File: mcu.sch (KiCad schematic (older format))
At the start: 28 parts, among them P1 CONN_01X02, SW1 SW_PUSH, T2 MMBT3904, U2 STM32F072CB, U6 24AA01, Y1 8MHz

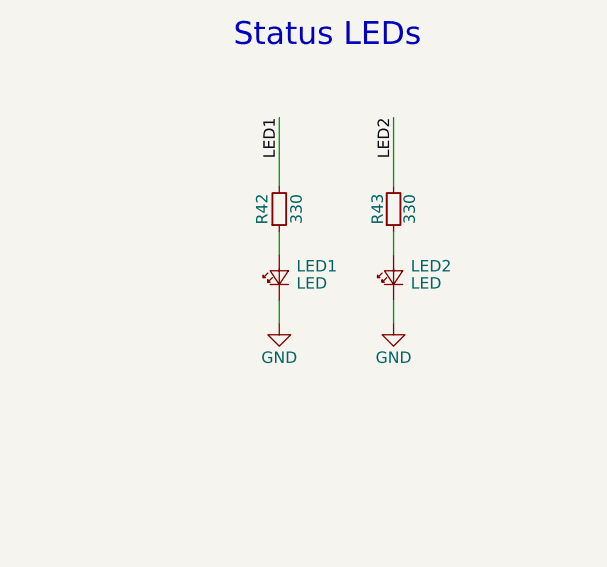
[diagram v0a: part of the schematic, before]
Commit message: BOM updated
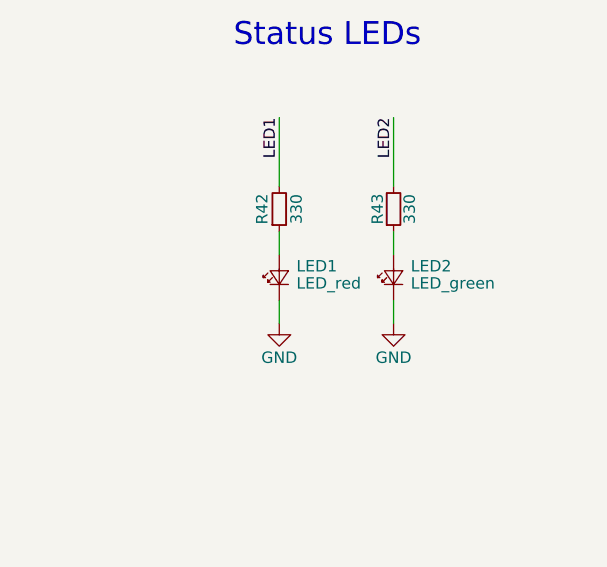
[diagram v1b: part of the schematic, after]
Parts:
- LED1: value LED -> LED_red
- LED2: value LED -> LED_green
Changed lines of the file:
@@
 AR Path="/58A68DCB/58AE11BD" Ref="LED2"  Part="1"
 F 0 "LED2" V 10150 5325 50  0000 R CNN
-F 1 "LED" V 10075 5325 50  0000 R CNN
+F 1 "LED_green" V 10075 5325 50  0000 R CNN
 F 2 "LEDs:LED_0603" V 10100 5400 50  0001 C CNN
 F 3 "" V 10100 5400 50  0001 C CNN
@@
 AR Path="/58A68DCB/58AE0EA3" Ref="LED1"  Part="1"
 F 0 "LED1" V 9650 5325 50  0000 R CNN
-F 1 "LED" V 9575 5325 50  0000 R CNN
+F 1 "LED_red" V 9575 5325 50  0000 R CNN
 F 2 "LEDs:LED_0603" V 9600 5400 50  0001 C CNN
 F 3 "" V 9600 5400 50  0001 C CNN

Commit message: Final version for Jan/2018 production
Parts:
- C33, C36: PartNumber GRM188R60J225KE19D -> GRM188R61E225KA12D; Remarks 6.3V, X5R -> 25V, X5R
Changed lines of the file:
@@
 Sheet 3 6
 Title "MPPT Charger 20A"
-Date "2017-12-11"
-Rev "0.9"
+Date "2018-01-18"
+Rev "0.10"
 Comp "Libre Solar"
 Comment1 "Author: Martin Jäger"
@@
 F 3 "" H 6050 4800 50  0000 C CNN
 F 4 "Murata" H 3600 -700 50  0001 C CNN "Manufacturer"
-F 5 "GRM188R60J225KE19D" H 3600 -700 50  0001 C CNN "PartNumber"
-F 6 "6.3V, X5R" H 0   0   60  0001 C CNN "Remarks"
+F 5 "GRM188R61E225KA12D" H 3600 -700 50  0001 C CNN "PartNumber"
+F 6 "25V, X5R" H 0   0   60  0001 C CNN "Remarks"
 	1    6050 4800
 	1    0    0    -1
@@
 F 3 "" H 9100 2700 50  0000 C CNN
 F 4 "Murata" H -250 0   50  0001 C CNN "Manufacturer"
-F 5 "GRM188R60J225KE19D" H -250 0   50  0001 C CNN "PartNumber"
-F 6 "6.3V, X5R" H 0   0   60  0001 C CNN "Remarks"
+F 5 "GRM188R61E225KA12D" H -250 0   50  0001 C CNN "PartNumber"
+F 6 "25V, X5R" H 0   0   60  0001 C CNN "Remarks"
 	1    9100 2700
 	1    0    0    -1
